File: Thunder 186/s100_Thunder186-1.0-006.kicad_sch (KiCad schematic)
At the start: 0 parts

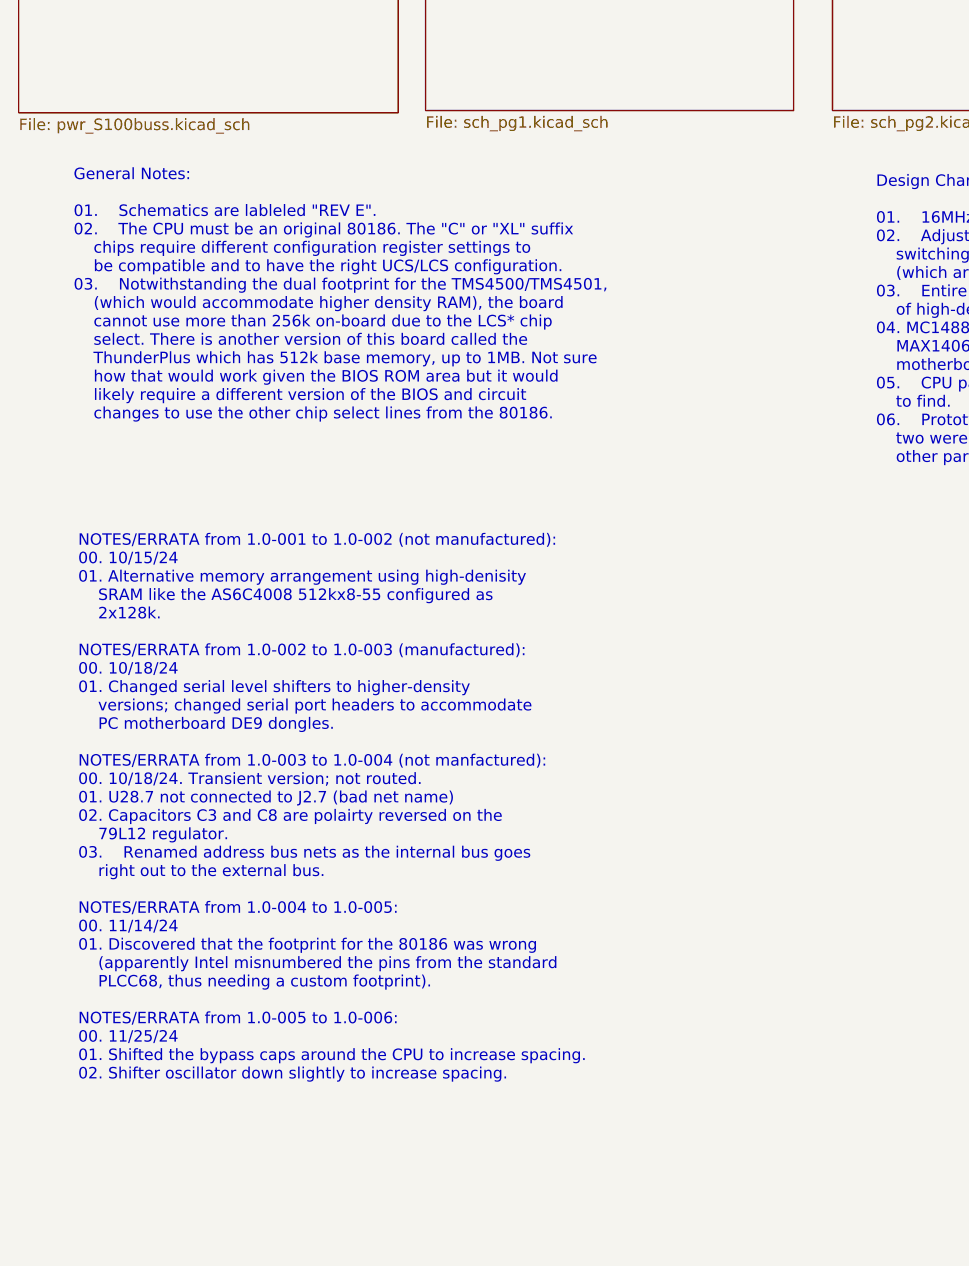
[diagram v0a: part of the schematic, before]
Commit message: Add files via upload
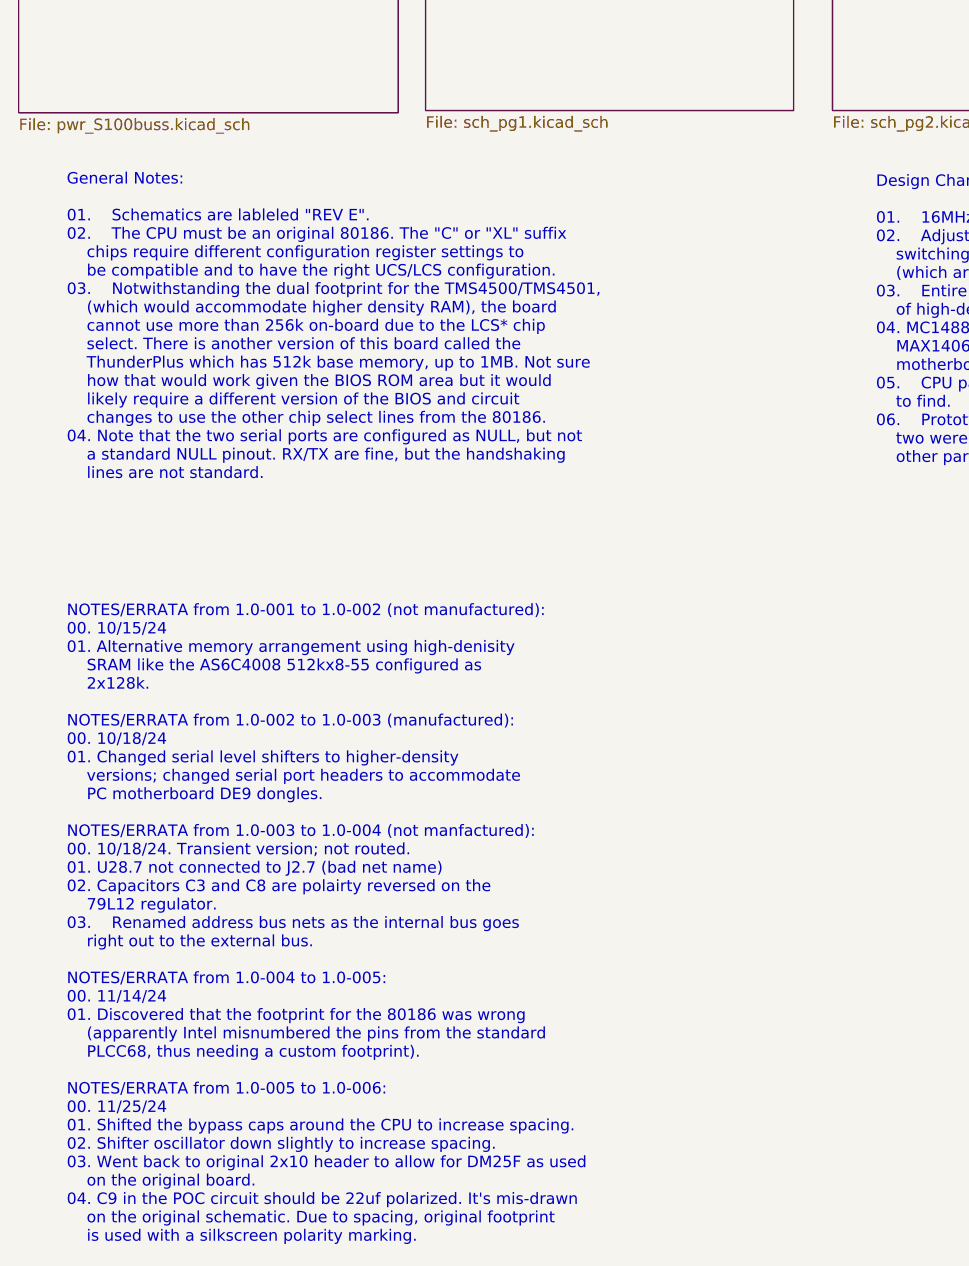
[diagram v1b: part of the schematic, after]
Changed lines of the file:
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@@
 	(title_block
 		(title "Lomas Thunder 186 Rev. E")
-		(date "2024-11-25")
+		(date "2024-11-28")
 		(rev "1.0-006")
 		(company "Lomas Data Produtcs")
@@
 		(comment 2 "Schematic page 1")
 	)
-	(text "General Notes:\n\n01.	Schematics are lableled \"REV E\".\n02.	The CPU must be an original 80186. The \"C\" or \"XL\" suffix\n	chips require different configuration register settings to\n	be compatible and to have the right UCS/LCS configuration.\n03.	Notwithstanding the dual footprint for the TMS4500/TMS4501,\n	(which would accommodate higher density RAM), the board\n	cannot use more than 256k on-board due to the LCS* chip\n	select. There is another version of this board called the\n	ThunderPlus which has 512k base memory, up to 1MB. Not sure\n	how that would work given the BIOS ROM area but it would\n	likely require a different version of the BIOS and circuit\n	changes to use the other chip select lines from the 80186.\n"
+	(text "General Notes:\n\n01.	Schematics are lableled \"REV E\".\n02.	The CPU must be an original 80186. The \"C\" or \"XL\" suffix\n	chips require different configuration register settings to\n	be compatible and to have the right UCS/LCS configuration.\n03.	Notwithstanding the dual footprint for the TMS4500/TMS4501,\n	(which would accommodate higher density RAM), the board\n	cannot use more than 256k on-board due to the LCS* chip\n	select. There is another version of this board called the\n	ThunderPlus which has 512k base memory, up to 1MB. Not sure\n	how that would work given the BIOS ROM area but it would\n	likely require a different version of the BIOS and circuit\n	changes to use the other chip select lines from the 80186.\n04. Note that the two serial ports are configured as NULL, but not\n	a standard NULL pinout. RX/TX are fine, but the handshaking \n	lines are not standard.\n"
 		(exclude_from_sim no)
-		(at 24.13 71.374 0)
+		(at 23.368 74.93 0)
 		(effects
 			(font
@@
 		)
 	)
-	(text "NOTES/ERRATA from 1.0-001 to 1.0-002 (not manufactured):\n00. 10/15/24\n01. Alternative memory arrangement using high-denisity\n    SRAM like the AS6C4008 512kx8-55 configured as\n	2x128k. \n\nNOTES/ERRATA from 1.0-002 to 1.0-003 (manufactured):\n00. 10/18/24\n01. Changed serial level shifters to higher-density\n	versions; changed serial port headers to accommodate\n	PC motherboard DE9 dongles.\n\nNOTES/ERRATA from 1.0-003 to 1.0-004 (not manfactured):\n00. 10/18/24. Transient version; not routed.\n01. U28.7 not connected to J2.7 (bad net name)\n02. Capacitors C3 and C8 are polairty reversed on the\n	79L12 regulator.\n03.	Renamed address bus nets as the internal bus goes\n	right out to the external bus.\n\nNOTES/ERRATA from 1.0-004 to 1.0-005:\n00. 11/14/24\n01. Discovered that the footprint for the 80186 was wrong\n	(apparently Intel misnumbered the pins from the standard\n	PLCC68, thus needing a custom footprint).\n\nNOTES/ERRATA from 1.0-005 to 1.0-006:\n00. 11/25/24\n01. Shifted the bypass caps around the CPU to increase spacing.\n02. Shifter oscillator down slightly to increase spacing.\n"
+	(text "NOTES/ERRATA from 1.0-001 to 1.0-002 (not manufactured):\n00. 10/15/24\n01. Alternative memory arrangement using high-denisity\n    SRAM like the AS6C4008 512kx8-55 configured as\n	2x128k. \n\nNOTES/ERRATA from 1.0-002 to 1.0-003 (manufactured):\n00. 10/18/24\n01. Changed serial level shifters to higher-density\n	versions; changed serial port headers to accommodate\n	PC motherboard DE9 dongles.\n\nNOTES/ERRATA from 1.0-003 to 1.0-004 (not manfactured):\n00. 10/18/24. Transient version; not routed.\n01. U28.7 not connected to J2.7 (bad net name)\n02. Capacitors C3 and C8 are polairty reversed on the\n	79L12 regulator.\n03.	Renamed address bus nets as the internal bus goes\n	right out to the external bus.\n\nNOTES/ERRATA from 1.0-004 to 1.0-005:\n00. 11/14/24\n01. Discovered that the footprint for the 80186 was wrong\n	(apparently Intel misnumbered the pins from the standard\n	PLCC68, thus needing a custom footprint).\n\nNOTES/ERRATA from 1.0-005 to 1.0-006:\n00. 11/25/24\n01. Shifted the bypass caps around the CPU to increase spacing.\n02. Shifter oscillator down slightly to increase spacing.\n03. Went back to original 2x10 header to allow for DM25F as used\n	on the original board.\n04. C9 in the POC circuit should be 22uf polarized. It's mis-drawn\n	on the original schematic. Due to spacing, original footprint\n	is used with a silkscreen polarity marking.\n"
 		(exclude_from_sim no)
-		(at 24.638 158.75 0)
+		(at 23.368 176.784 0)
 		(effects
 			(font
@@
 			)
 			(justify left bottom)
-			(href "#1")
 		)
 	)
